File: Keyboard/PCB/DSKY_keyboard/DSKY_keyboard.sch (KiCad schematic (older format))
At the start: 54 parts, among them J1 Conn_01x04_Male, J2 MOUNTINGHOLE3.0, J3 MOUNTINGHOLE3.0, J4 MOUNTINGHOLE3.0, J5 MOUNTINGHOLE3.0, SW1 SW_SPST_LED, SW10 SW_SPST_LED, SW11 SW_SPST_LED, SW12 SW_SPST_LED, SW13 SW_SPST_LED, SW14 SW_SPST_LED, SW15 SW_SPST_LED, SW16 SW_SPST_LED, SW17 SW_SPST_LED, SW18 SW_SPST_LED, SW19 SW_SPST_LED, SW2 SW_SPST_LED, SW20 SWITCH_TACT_SMT4.6X2.8, SW3 SW_SPST_LED, SW4 SW_SPST_LED, SW5 SW_SPST_LED, SW6 SW_SPST_LED, SW7 SW_SPST_LED, SW8 SW_SPST_LED, SW9 SW_SPST_LED, U1 STM32F042K6T6, U2 AQY232SZ, U3 AP2112K-3.3

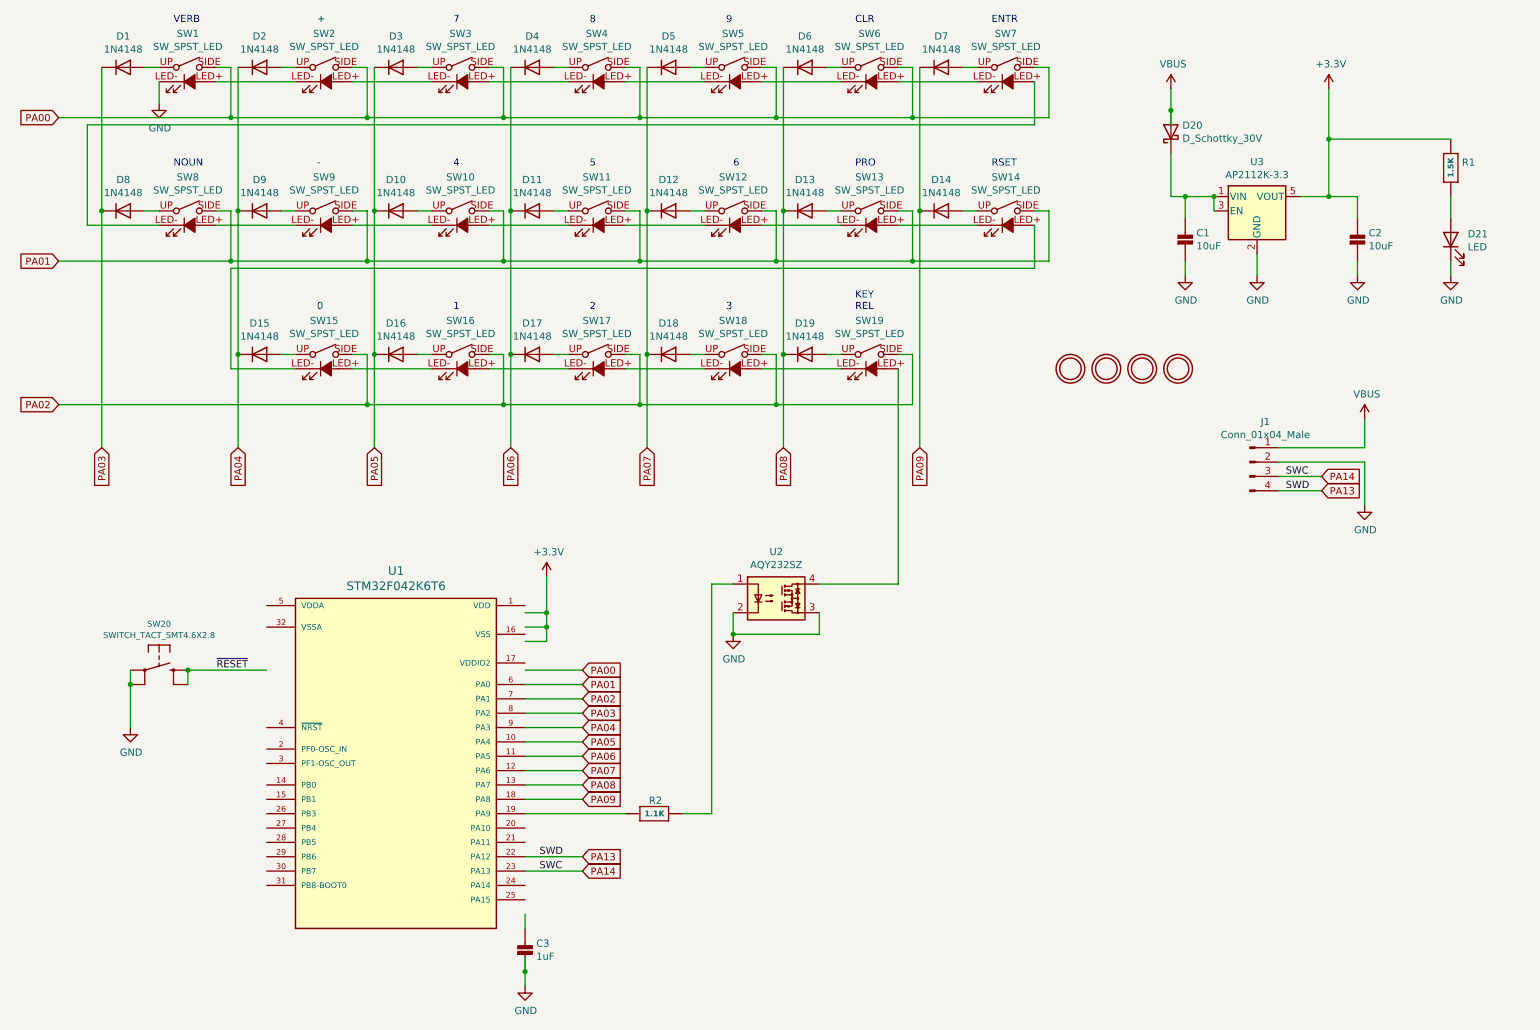
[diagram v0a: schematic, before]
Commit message: PCB updates
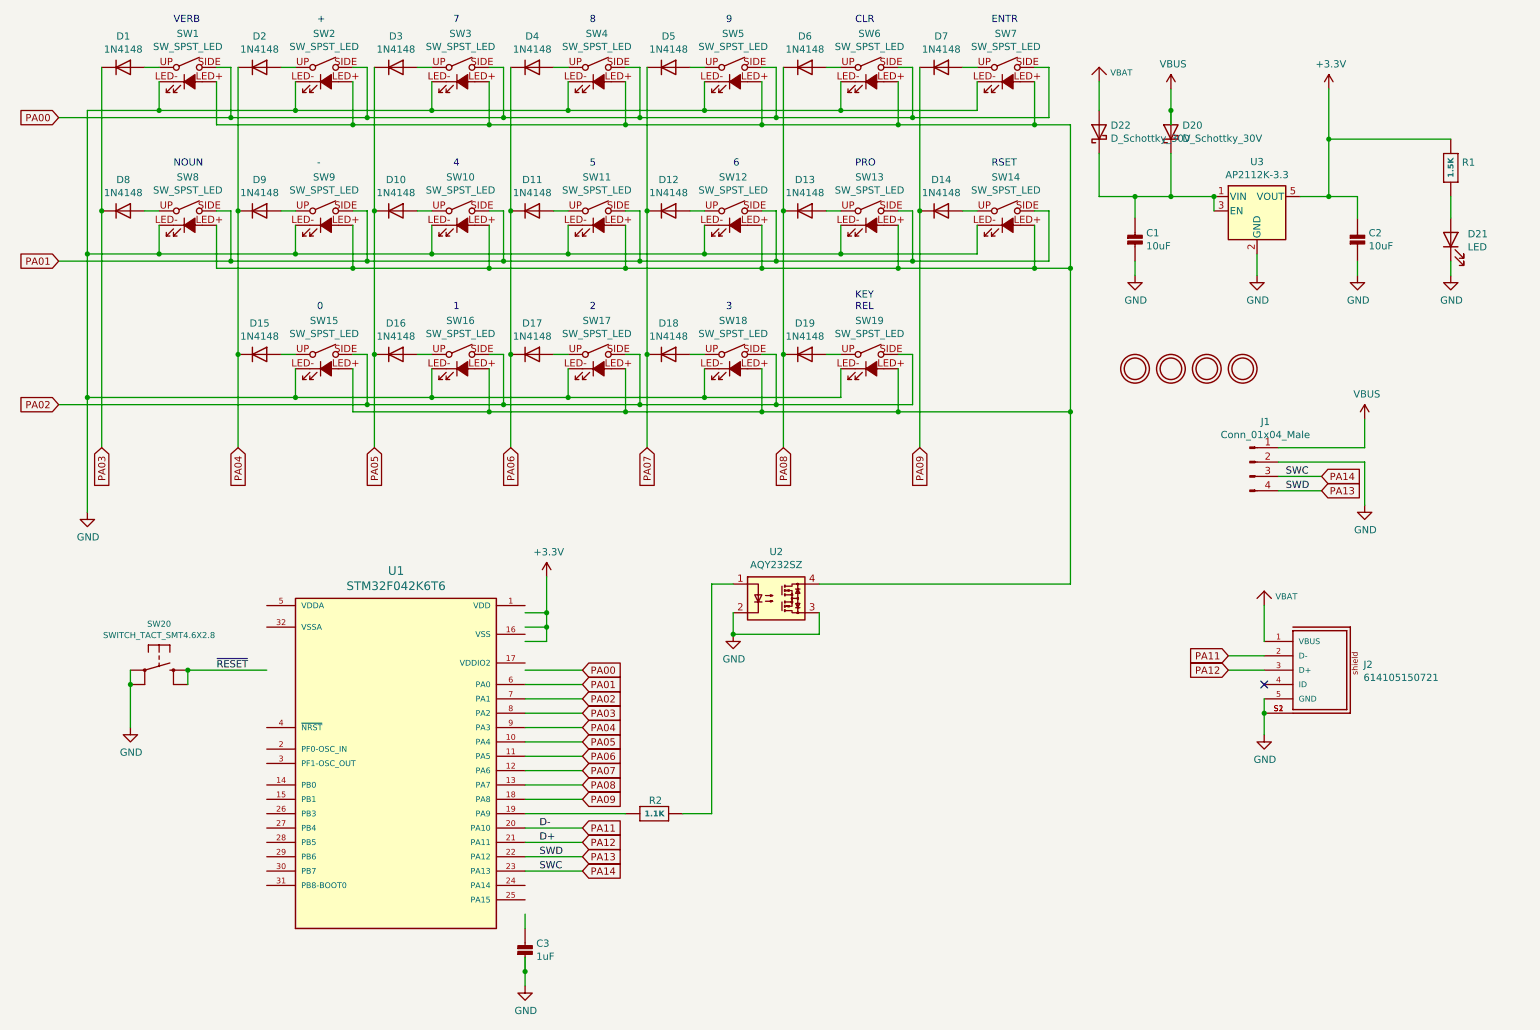
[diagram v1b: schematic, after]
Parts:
- added D22: D_Schottky_30V, Trinket M0 rev D:SOD-123FL, symbol Device:D_Schottky
- added J2: 614105150721, Footprints:614105150721, symbol 614105150721:614105150721
- J3: renamed from J2; footprint (none) -> Trinket M0 rev D:MOUNTINGHOLE_2.0_PLATED
- J4: renamed from J3; footprint (none) -> Trinket M0 rev D:MOUNTINGHOLE_2.0_PLATED
- J5: renamed from J4; footprint (none) -> Trinket M0 rev D:MOUNTINGHOLE_2.0_PLATED
- J6: renamed from J5; footprint (none) -> Trinket M0 rev D:MOUNTINGHOLE_2.0_PLATED
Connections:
- net labels added: D+, D-, PA11, PA12, VBAT
- wire segments 178 -> 244
- no-connect marks 0 -> 1
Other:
- moved on the sheet: C1

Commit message: Update
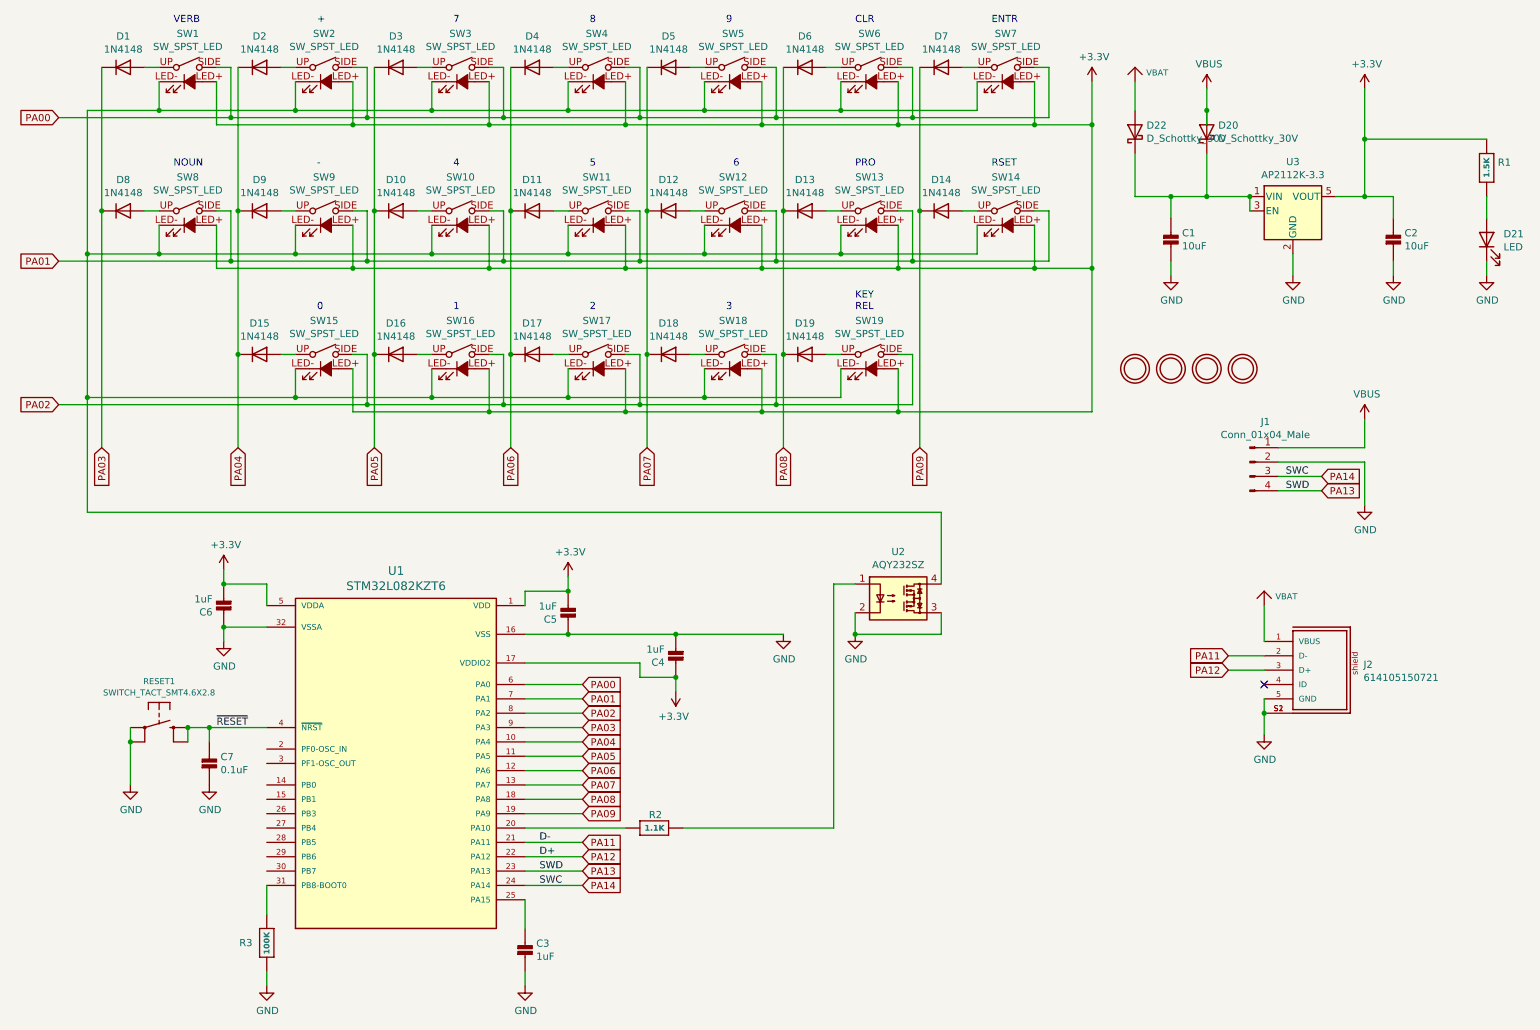
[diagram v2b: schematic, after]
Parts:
- added C4, C5, C6: 1uF, Trinket M0 rev D:0603-NO, symbol Trinket_M0_rev_D-eagle-import:CAP_CERAMIC0805-NOOUTLINE
- added C7: 0.1uF, Trinket M0 rev D:0603-NO, symbol Trinket_M0_rev_D-eagle-import:CAP_CERAMIC0805-NOOUTLINE
- added R3: 100K, Trinket M0 rev D:0603-NO, symbol Trinket_M0_rev_D-eagle-import:RESISTOR_0603_NOOUT
- U1: value STM32F042K6T6 -> STM32L082KZT6
- renumbered SW20 to RESET1
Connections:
- wire segments 244 -> 257
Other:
- moved on the sheet: C1, C2, D20, D21, D22, R1, R2, RESET1, U2, U3
